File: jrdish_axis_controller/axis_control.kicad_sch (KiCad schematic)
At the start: 25 parts, among them CN1 KF2EDGR-2.54-9P, CN2 KF2EDGR-2.54-6P

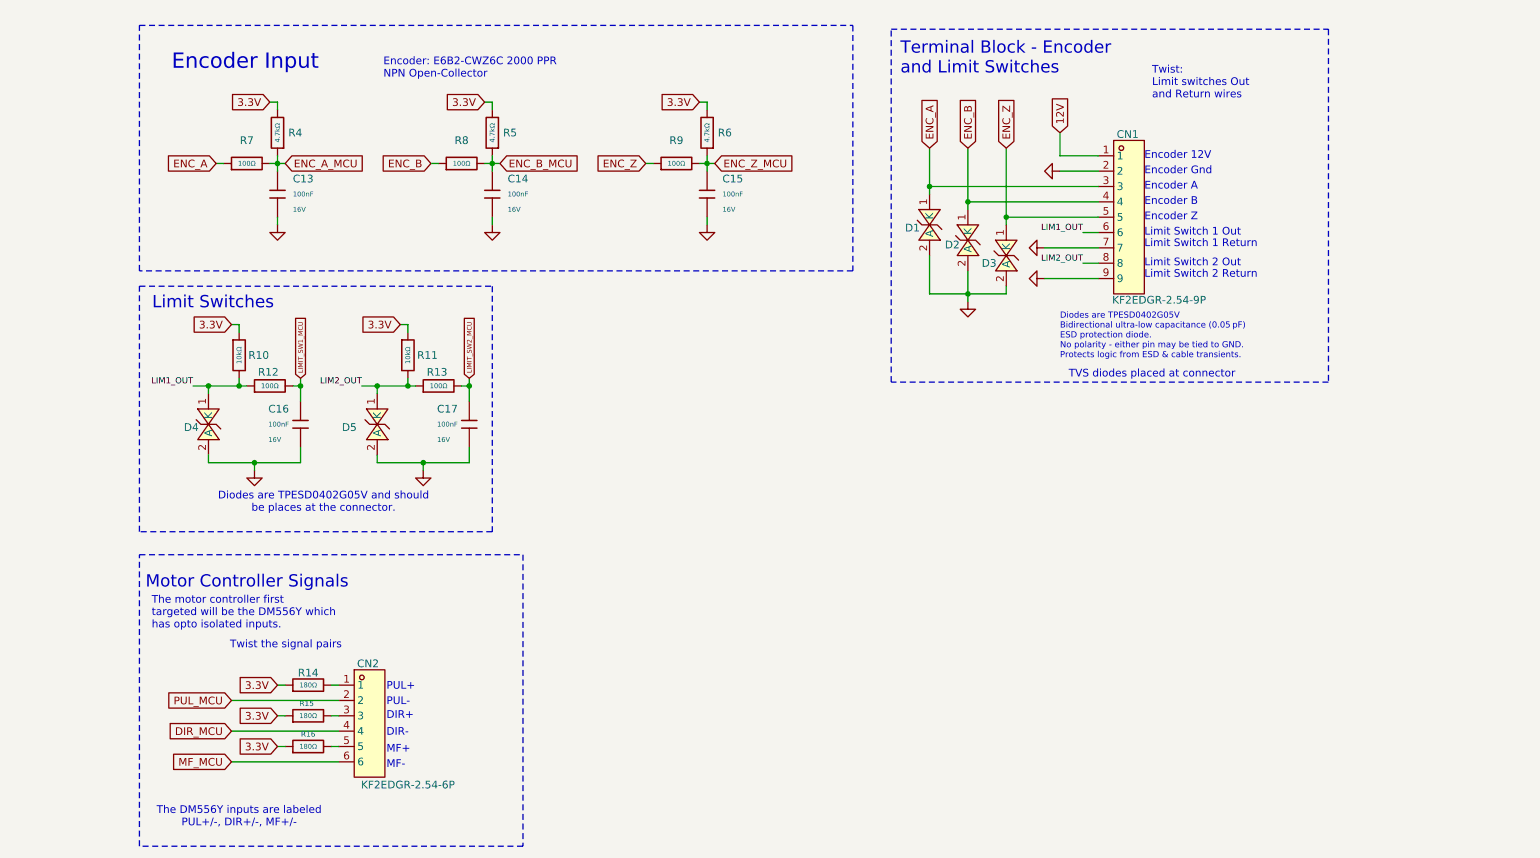
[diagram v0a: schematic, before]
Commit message: PCB layout in progress
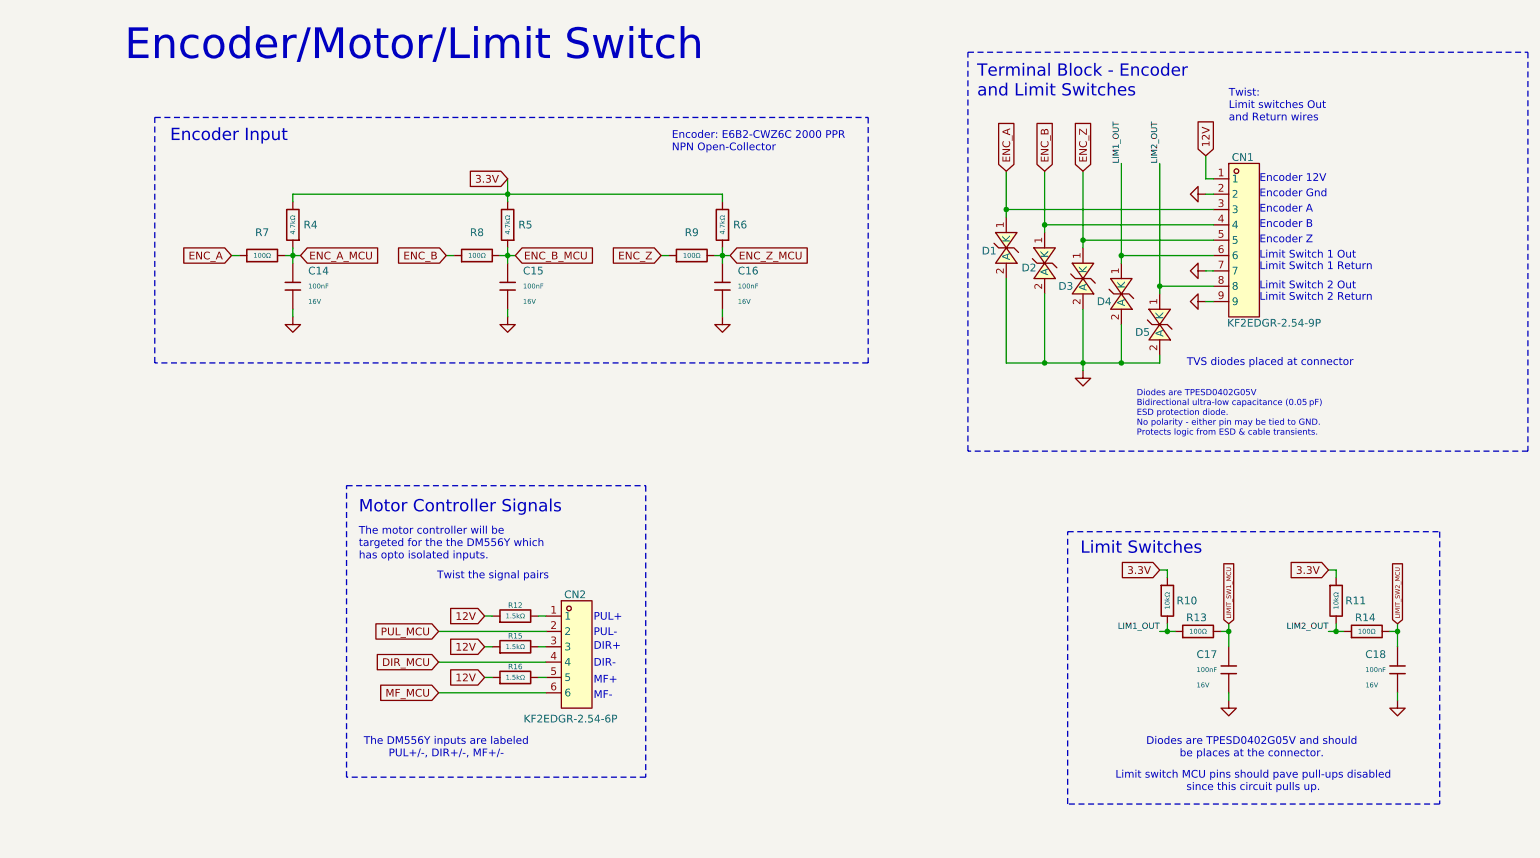
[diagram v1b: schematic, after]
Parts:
- removed R14, R15, R16: 180Ω, PCM_JLCPCB:R_0603, symbol PCM_JLCPCB-Resistors:0603,180Ω
- added R12, R15, R16: 1.5kΩ, PCM_JLCPCB:R_0402, symbol PCM_JLCPCB-Resistors:0402,1.5kΩ
- renumbered C13 to C14, C14 to C15, C15 to C16, C16 to C17, C17 to C18, R12 to R13, R13 to R14
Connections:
- net 12V: now also R12.1, R15.1, R16.1
- net at CN2.5: now also R16.2
- net at CN2.1: now also R12.2
- net at CN2.3: now also R15.2
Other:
- note added: "Encoder/Motor/Limit Switch"
- note added: "Limit switch MCU pins should pave pull-ups disabled since this circuit pulls up."
- note added: "The motor controller will be targeted for the the DM556Y which has opto isolated inputs."
- note removed: "The motor controller first targeted will be the DM556Y which has opto isolated inputs."
- company: (none) -> JRSeti
- title: (none) -> Encoder/Motor/Limit Switch
- moved on the sheet: C14, C15, C16, C17, C18, CN1, CN2, D1, D2, D3, R10, R11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
